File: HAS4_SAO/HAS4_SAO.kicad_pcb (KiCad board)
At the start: 2 copper layers, 5 parts, among them SW1 MLL1200S, X1 Badgelife_sao_connector_v169b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

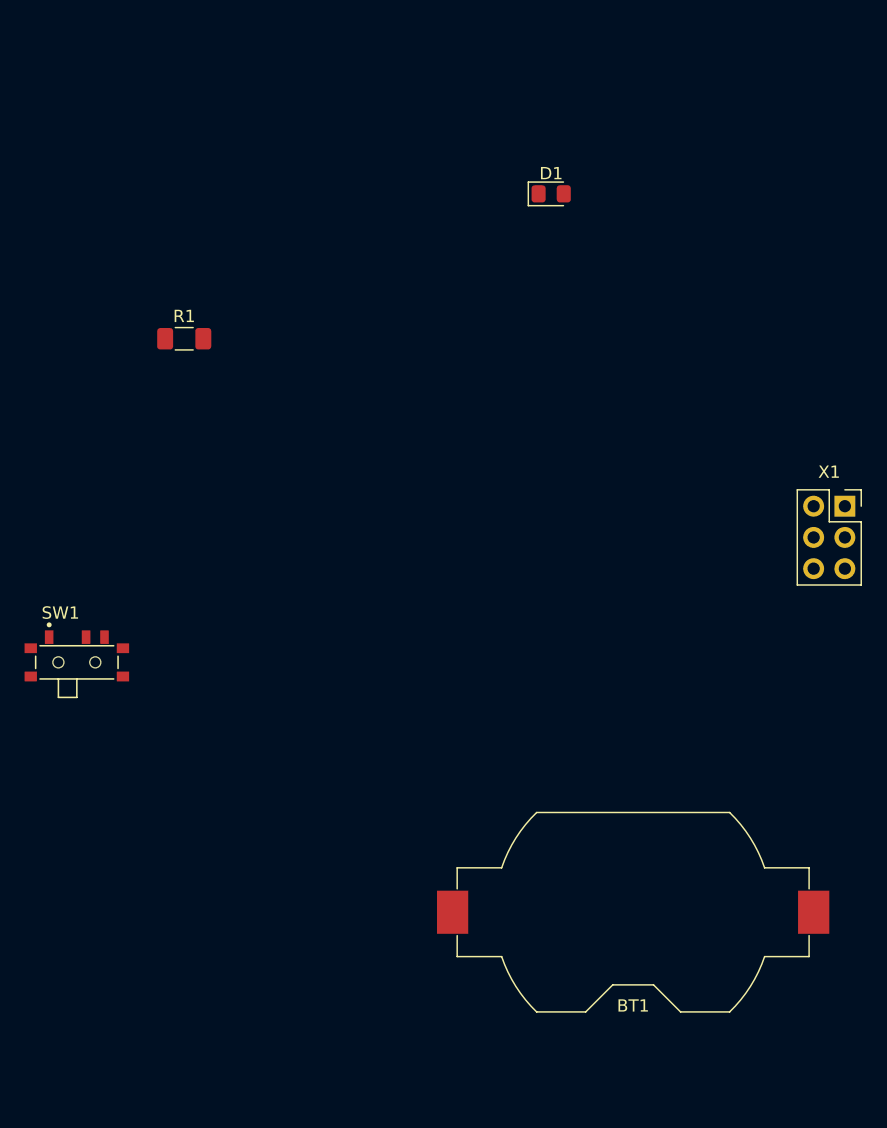
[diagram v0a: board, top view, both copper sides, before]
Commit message: HAS4 SAO work
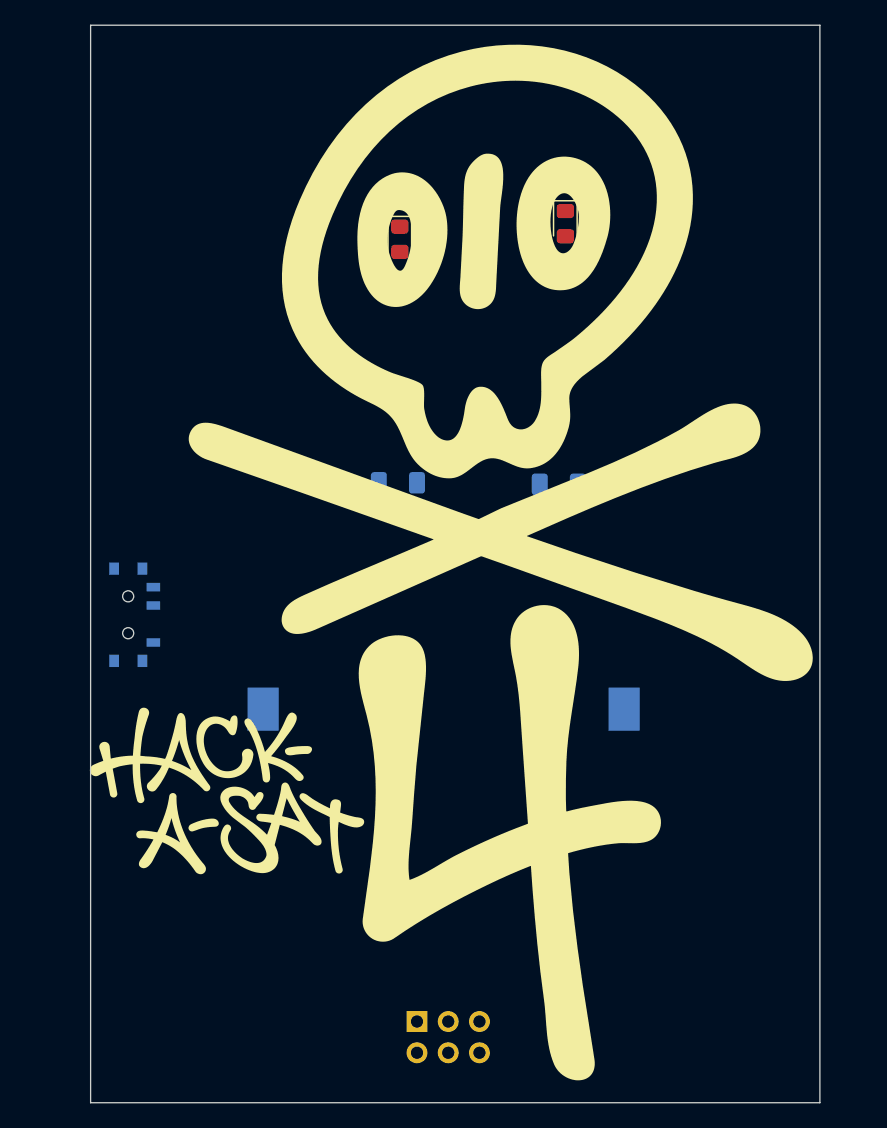
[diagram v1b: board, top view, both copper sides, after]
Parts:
- added D2: LED, LED_SMD:LED_0805_2012Metric_Pad1.15x1.40mm_HandSolder, F.Cu at (103.5, 64.7)
- added R2: R, Resistor_SMD:R_1206_3216Metric_Pad1.30x1.75mm_HandSolder, B.Cu at (103.4, 84.5)
- BT1, R1, SW1: moved to B.Cu
- X1: footprint Connector_PinSocket_2.54mm:PinSocket_2x03_P2.54mm_Vertical -> Connector_PinHeader_2.54mm:PinHeader_2x03_P2.54mm_Vertical; moved to B.Cu
- moved X1 54.5 mm to (104.9, 128.3), turned to -90 degrees
- moved R1 32.7 mm to (116.4, 84.6), turned to 180 degrees
- moved BT1 22.6 mm to (107.1, 102.9), turned to 180 degrees
- moved SW1 5.69 mm to (81.4, 95.2), turned to 90 degrees
- moved D1 2.68 mm to (117.0, 63.4), turned to -90 degrees
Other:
- board outline added: 59.3 x 87.6 mm
- board text added: "Glue pin here or wherever"

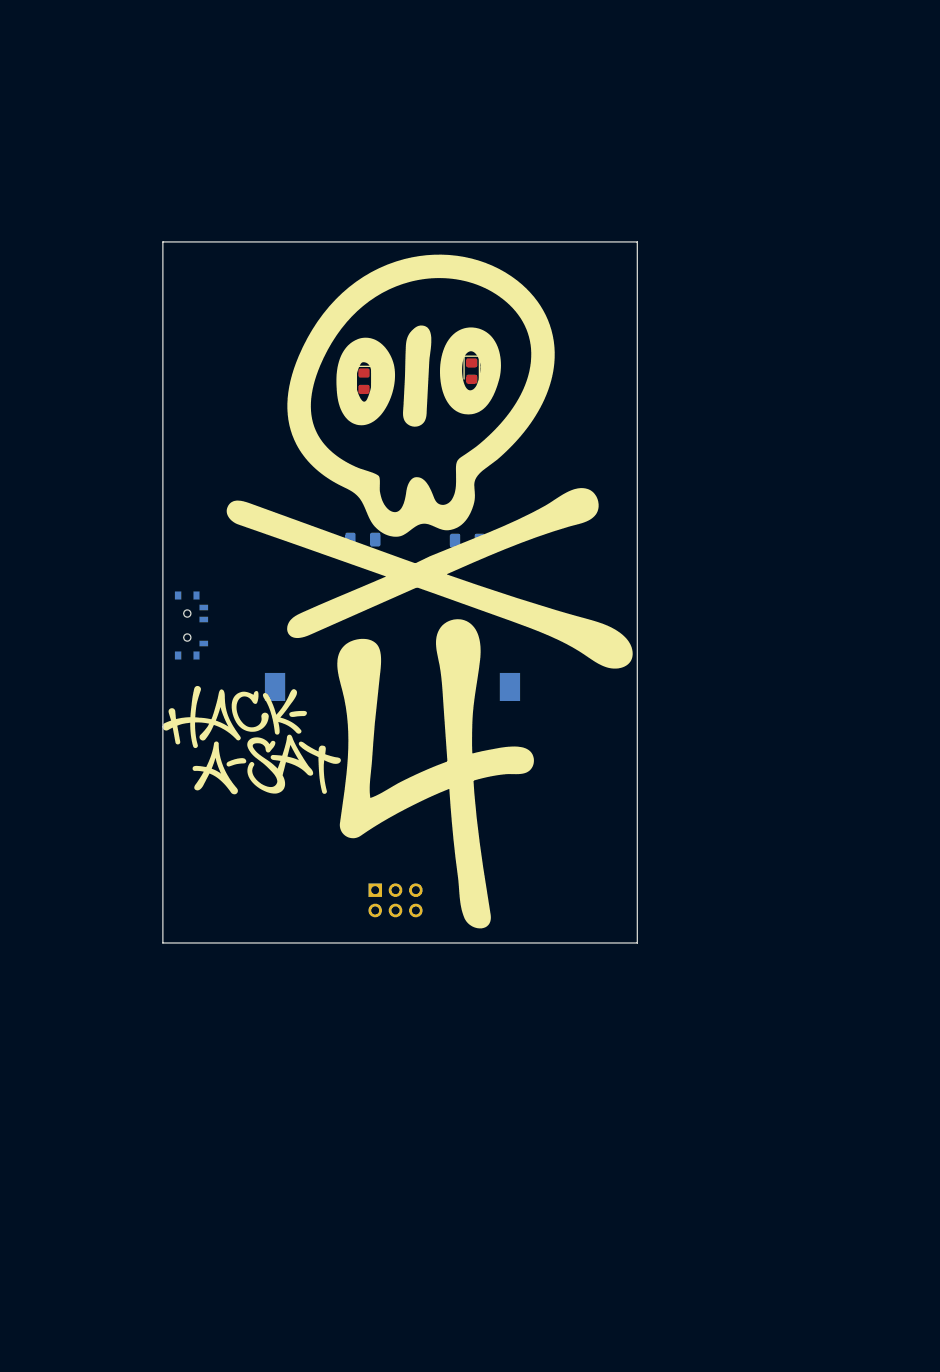
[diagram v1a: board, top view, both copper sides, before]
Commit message: HAS4 SAO for DC31
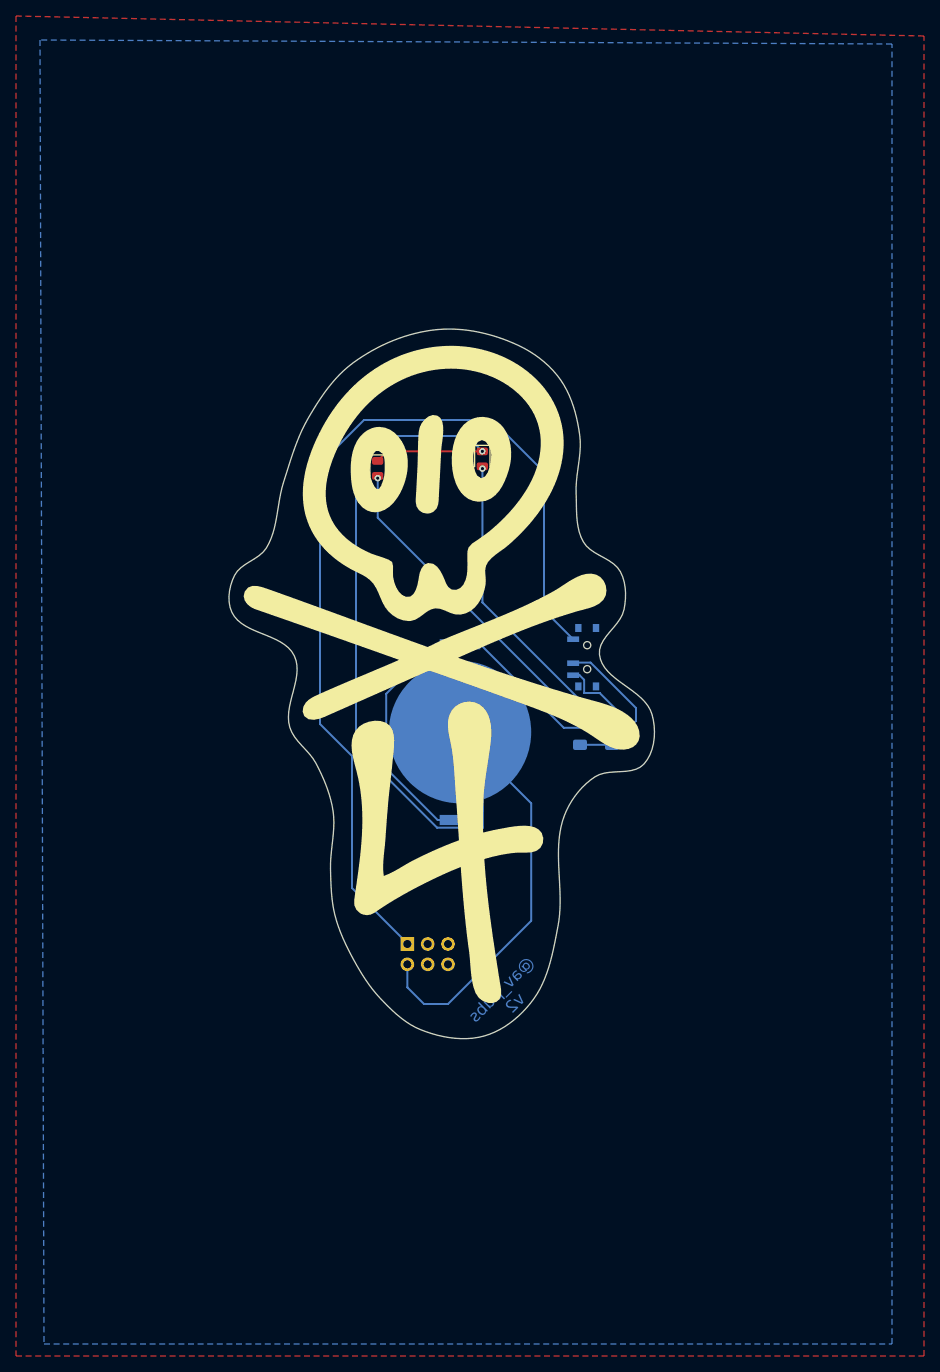
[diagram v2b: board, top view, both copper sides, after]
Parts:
- removed X1: Badgelife_sao_connector_v169bis, Connector_PinHeader_2.54mm:PinHeader_2x03_P2.54mm_Vertical
- added J1: Conn_02x03_Counter_Clockwise, Connector_PinHeader_2.54mm:PinHeader_2x03_P2.54mm_Vertical, B.Cu at (108.9, 135.0)
- added svg2mod: G***, HAS4_images:HAS4_bug, F.Cu at (113.2, 102.5)
- BT1: footprint Battery:BatteryHolder_Keystone_1058_1x2032 -> Battery:BatteryHolder_Keystone_3034_1x20mm
- D1, D2: footprint LED_SMD:LED_0805_2012Metric_Pad1.15x1.40mm_HandSolder -> LED_SMD:LED_0805_2012Metric
- SW1: value MLL1200S -> SW_SPDT; footprint MLL1200S:SW_MLL1200S -> Button_Switch_SMD:SW_SPDT_PCM12
- moved SW1 49.8 mm to (131.1, 99.2), turned to -90 degrees
- moved R2 36.3 mm to (130.5, 108.5), turned to 90 degrees
- moved R1 30.0 mm to (134.5, 108.5), turned to 90 degrees
- moved D1 11.1 mm to (118.3, 74.4)
- moved D2 11.0 mm to (105.2, 75.6)
- moved BT1 10.2 mm to (115.5, 108.5), turned to 90 degrees
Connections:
- SW1 pad 1: Net-(BT1-+) -> Net-(J1-Pin_1)
- SW1 pad 3: Net-(X1-VCC) -> Net-(BT1-+)
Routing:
- net GND: track 0.00 -> 152.1 mm, vias 0 -> 1
- net Net-(J1-Pin_1): track 0.00 -> 119.9 mm
- net Net-(BT1-+): track 0.00 -> 68.0 mm
- net Net-(D2-A): track 0.00 -> 41.0 mm, vias 0 -> 1
- net Net-(D1-A): track 0.00 -> 39.3 mm, vias 0 -> 1
- net Net-(SW1-B): track 0.00 -> 20.1 mm
- added copper zone on B.Cu, net (none)
- added copper zone on F.Cu, net (none)
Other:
- board size 59.3 x 87.6 mm -> 53.2 x 88.7 mm
- board text added: "@av_pubs v2"
- board text added: "Batt pwr"
- board text added: "SAO pwr"
